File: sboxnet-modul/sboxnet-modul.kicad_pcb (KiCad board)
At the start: 2 copper layers, 62 x 62.4 mm, 39 parts, among them J1 Conn_01x03, J2 Conn_02x03_Odd_Even, J3 Conn_01x04_Female, J4 8P8C, J5 8P8C, J6 sboxnet-buchse_2x17, SW1 SW_Push, U1 MCP1703A-3302_SOT223, U2 MCP1703A-5002_SOT223, U3 SN65HVD230, U4 ATxmega128A4U-AU, Y1 16MHz

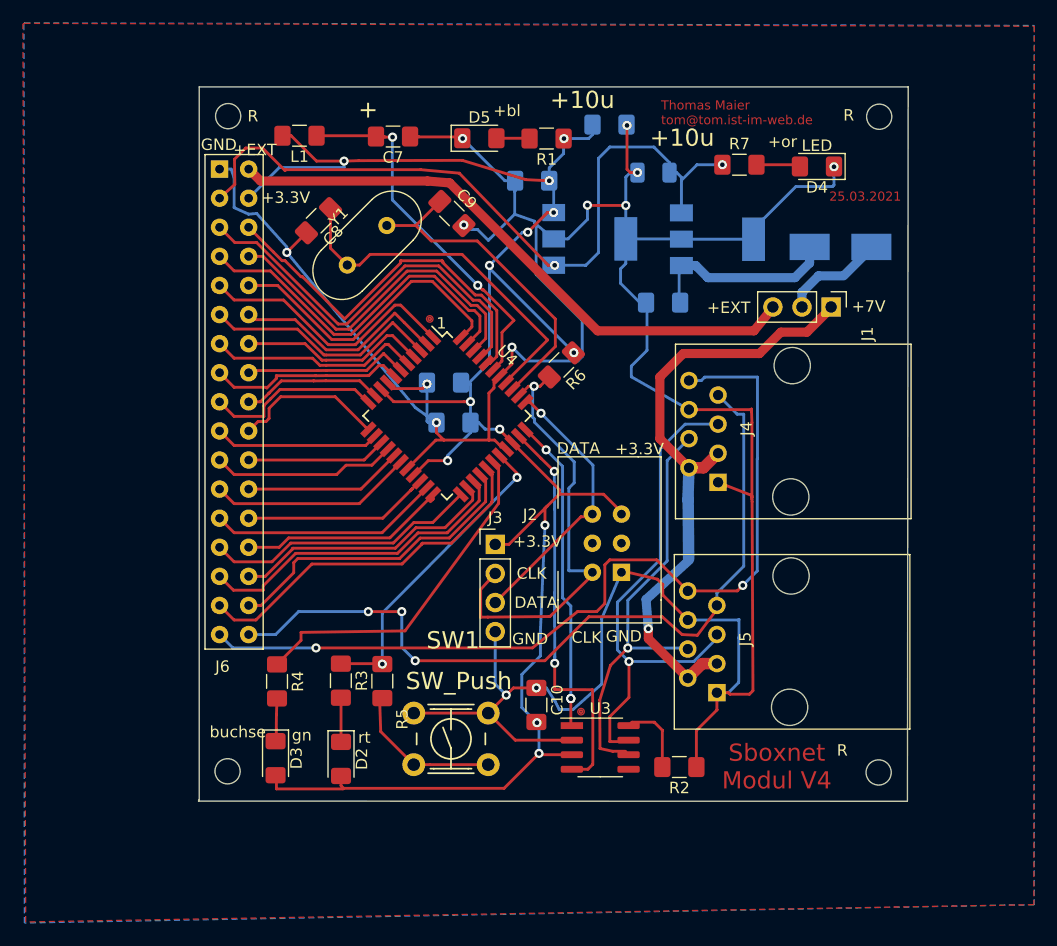
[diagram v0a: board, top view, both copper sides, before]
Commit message: sboxnet-modul v5
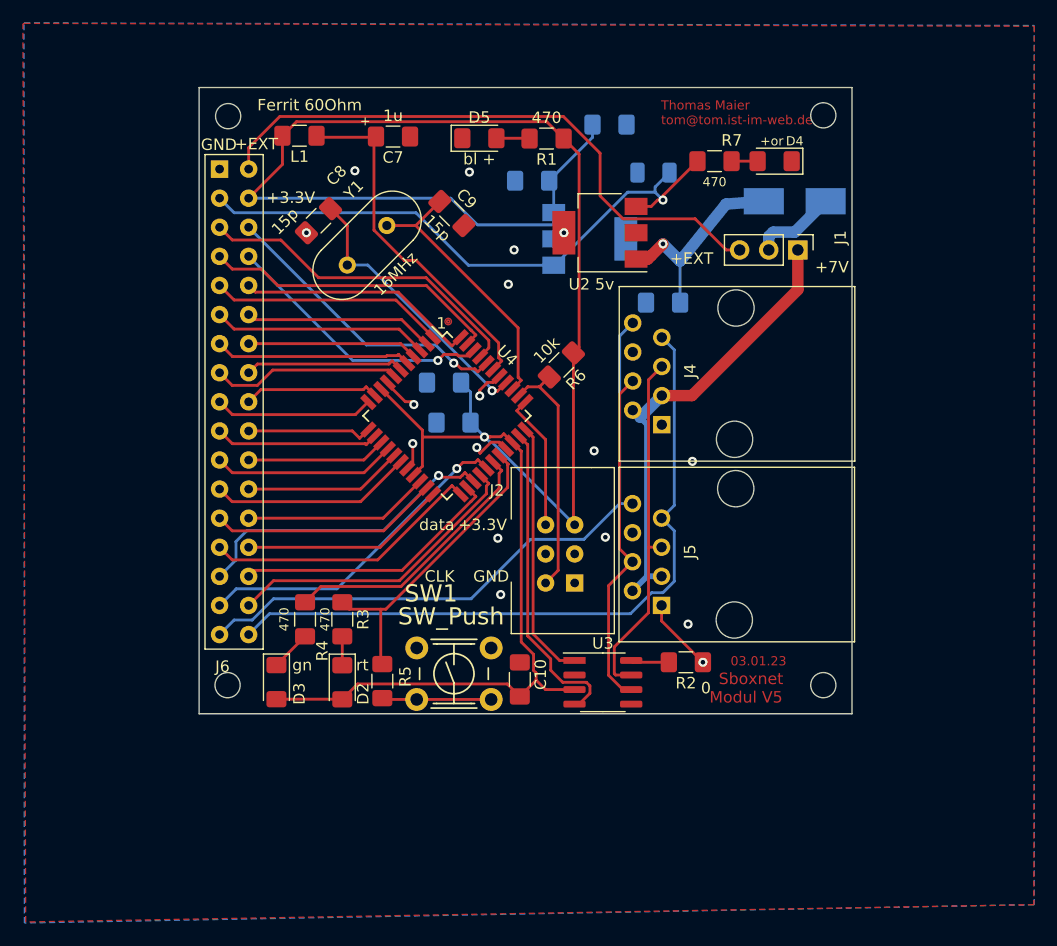
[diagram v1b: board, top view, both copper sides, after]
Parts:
- removed J3: Conn_01x04_Female, Connector_PinHeader_2.54mm:PinHeader_1x04_P2.54mm_Vertical
- C3: value 10u -> +10u
- D5: value LED -> bl +
- U1 3.3v: renamed from U1
- U2 5v: renamed from U2; moved to F.Cu
- moved U2 5v 10.3 mm to (126.8, 81.2), turned to 180 degrees
- moved R2 9.17 mm to (134.2, 118.8)
- moved J5 9.02 mm to (138.5, 109.3)
- moved Rx3 9.02 mm to (146.2, 120.8)
- moved buchse 7.52 mm to (94.2, 120.8)
- moved J4 7.03 mm to (138.5, 93.6)
- moved D2 6.69 mm to (104.2, 120.5)
- moved D3 6.64 mm to (98.5, 120.5)
- moved R4 5.95 mm to (101.0, 115.0)
- moved J1 5.76 mm to (144.0, 82.8)
- moved SW1 5.70 mm to (114.0, 119.8)
- moved U3 5.69 mm to (127.0, 120.5)
- moved D1 5.65 mm to (143.8, 78.5)
- moved R3 5.36 mm to (104.2, 115.0)
- moved Rx2 4.88 mm to (146.2, 71.0)
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- renumbered R to Rx1, R to Rx2, R to Rx3
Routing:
- net GND: track 275.8 -> 18.9 mm, vias 13 -> 17
- net DCC_B: track 77.3 -> 57.0 mm, vias 2 -> 0
- net +3V3: track 171.1 -> 188.9 mm, vias 13 -> 1
- net PDICLK: track 38.8 -> 21.6 mm, vias 1 -> 0
- net +7V: track 54.3 -> 40.0 mm, vias 1 -> 0
- net CANH: track 44.7 -> 31.2 mm, vias 1 -> 0
- net +5V: track 65.7 -> 53.5 mm, vias 2 -> 1
- net PDI_DATA: track 23.9 -> 12.1 mm, vias 1 -> 0
- net CANL: track 38.0 -> 30.0 mm, vias 1 -> 0
- net PA0: track 34.2 -> 26.3 mm, vias 0 -> 1
- net DCC_A: track 69.6 -> 61.8 mm, vias 3 -> 0
- net Net-(C8-Pad1): track 31.8 -> 24.3 mm, vias 0 -> 1
- net Net-(U3-Pad4): track 35.3 -> 28.0 mm, vias 2 -> 0
- net PA2: track 30.6 -> 23.9 mm, vias 0 -> 1
- net PE0: track 30.3 -> 23.8 mm
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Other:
- board size 62 x 62.4 mm -> 57 x 54.7 mm
- board text added: "03.01.23"
- board text added: "Sboxnet Modul V5"
- board text added: "data"
- board text removed: "+bl"
- board text removed: "25.03.2021"
- board text removed: "DATA"
- board text removed: "Sboxnet Modul V4"

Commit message: restruktur
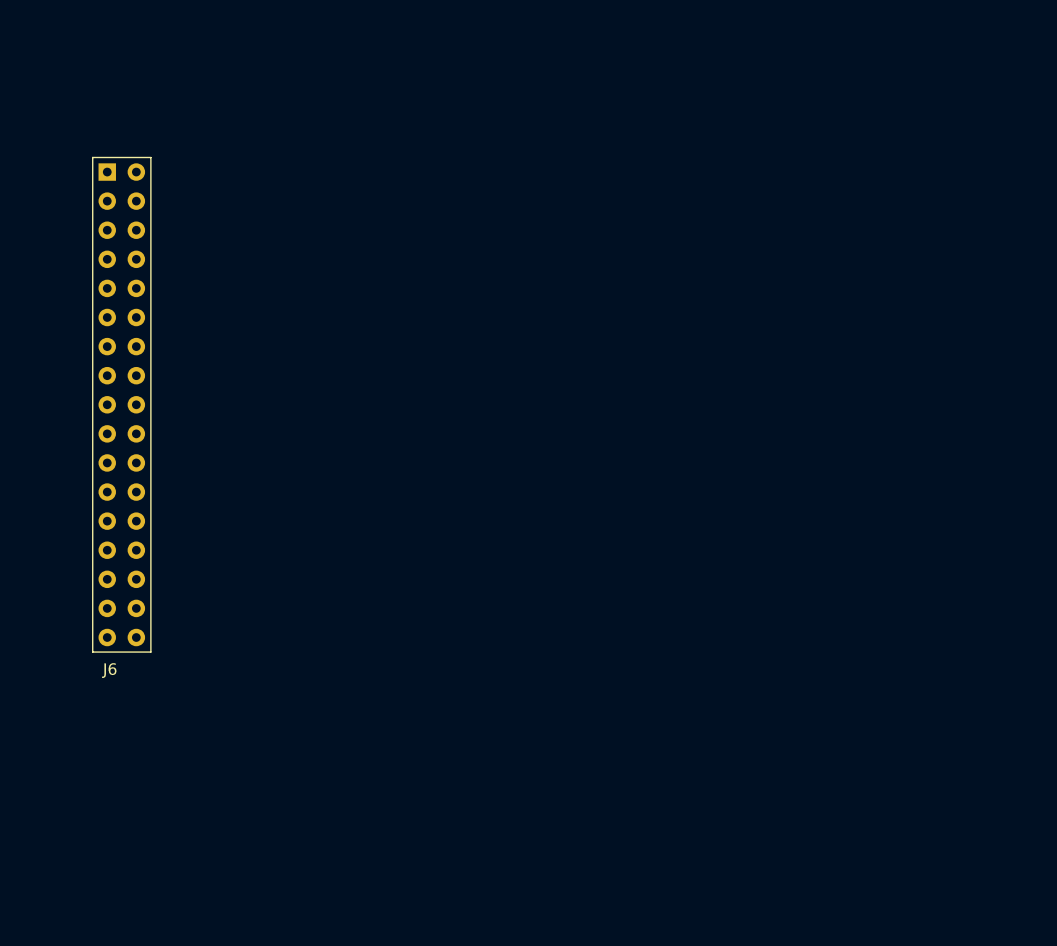
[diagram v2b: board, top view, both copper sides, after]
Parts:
- removed C1, C10, C4, C5, C6: 100n, Capacitor_SMD:C_1206_3216Metric_Pad1.42x1.75mm_HandSolder
- removed C2: 10u, Capacitor_SMD:C_1206_3216Metric_Pad1.42x1.75mm_HandSolder
- removed C3: +10u, Capacitor_SMD:C_1206_3216Metric
- removed C7: 1u, Capacitor_SMD:C_1206_3216Metric_Pad1.42x1.75mm_HandSolder
- removed C8, C9: 15p, Capacitor_SMD:C_1206_3216Metric_Pad1.42x1.75mm_HandSolder
- removed D1: SKL13B, Diode_SMD:D_SMB_Handsoldering
- removed D2, D3, D4: LED, LED_SMD:LED_1206_3216Metric_Pad1.42x1.75mm_HandSolder
- removed D5: bl +, LED_SMD:LED_1206_3216Metric_Pad1.42x1.75mm_HandSolder
- removed J1: Conn_01x03, Connector_PinHeader_2.54mm:PinHeader_1x03_P2.54mm_Vertical
- removed J2: Conn_02x03_Odd_Even, sboxnet:wannenstecker_gerade_6pin
- removed J4, J5: 8P8C, sboxnet:8p8c-mebp
- removed L1: Ferrit 60Ohm, Inductor_SMD:L_1206_3216Metric_Pad1.42x1.75mm_HandSolder
- removed R1, R3, R4, R7: 470, Resistor_SMD:R_1206_3216Metric_Pad1.42x1.75mm_HandSolder
- removed R2: 0, Resistor_SMD:R_1206_3216Metric_Pad1.42x1.75mm_HandSolder
- removed R5: 1k, Resistor_SMD:R_1206_3216Metric_Pad1.42x1.75mm_HandSolder
- removed R6: 10k, Resistor_SMD:R_1206_3216Metric_Pad1.42x1.75mm_HandSolder
- removed Rx1, Rx2, Rx3, buchse: MH2.2, MountingHole:MountingHole_2.2mm_M2
- removed SW1: SW_Push, sboxnet:JTP-1130
- removed U1 3.3v: MCP1703A-3302_SOT223, Package_TO_SOT_SMD:SOT-223-3_TabPin2
- removed U2 5v: MCP1703A-5002_SOT223, Package_TO_SOT_SMD:SOT-223-3_TabPin2
- removed U3: SN65HVD230, Package_SO:SOIC-8_3.9x4.9mm_P1.27mm
- removed U4: ATxmega128A4U-AU, Package_QFP:TQFP-44_10x10mm_P0.8mm
- removed Y1: 16MHz, Crystal:Crystal_HC49-U_Vertical
- moved J6 9.81 mm to (86.3, 119.1)
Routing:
- net +3V3: track 188.9 -> 0.00 mm, vias 1 -> 0
- net DCC_A: track 61.8 -> 0.00 mm
- net DCC_B: track 57.0 -> 0.00 mm
- net +5V: track 53.5 -> 0.00 mm, vias 1 -> 0
- net +V: track 52.9 -> 0.00 mm
- net +7V: track 40.0 -> 0.00 mm
- net CANH: track 31.2 -> 0.00 mm
- net AVCC: track 31.2 -> 0.00 mm
- net CANL: track 30.0 -> 0.00 mm
- net PA1: track 29.3 -> 0.00 mm
- net PD7: track 28.9 -> 0.00 mm, vias 1 -> 0
- net Net-(U3-Pad4): track 28.0 -> 0.00 mm
- net PD5: track 27.3 -> 0.00 mm, vias 1 -> 0
- net PE1: track 27.0 -> 0.00 mm
- net PD6: track 26.8 -> 0.00 mm
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- removed copper zone on B.Cu, net GND
- removed copper zone on F.Cu, net GND
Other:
- board outline removed
- board text removed: "+"
- board text removed: "+10u"
- board text removed: "+3.3V"
- board text removed: "+7V"
- board text removed: "+EXT"
- board text removed: "+or"
- board text removed: "03.01.23"
- board text removed: "1"
- board text removed: "CLK"
- board text removed: "GND"
- board text removed: "Sboxnet Modul V5"
- board text removed: "Thomas Maier tom@tom.ist-im-web.de"
- board text removed: "data"
- board text removed: "gn"
- board text removed: "rt"
